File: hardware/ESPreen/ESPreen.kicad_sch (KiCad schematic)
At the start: 4 parts

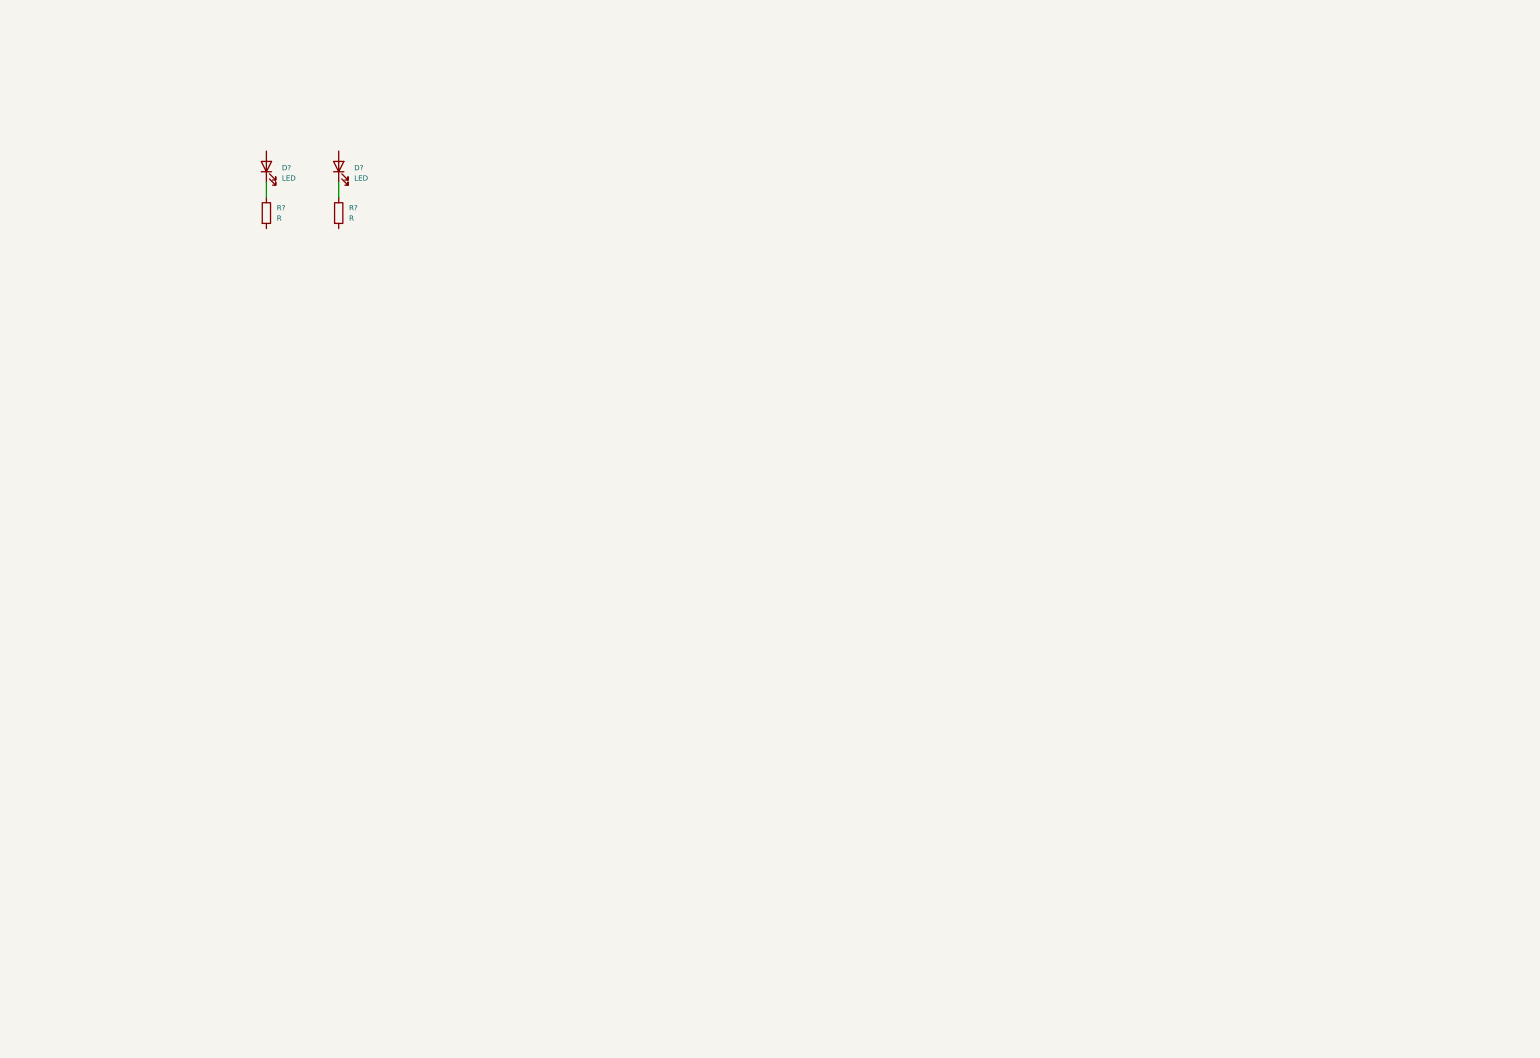
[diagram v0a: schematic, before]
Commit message: Update to finished board
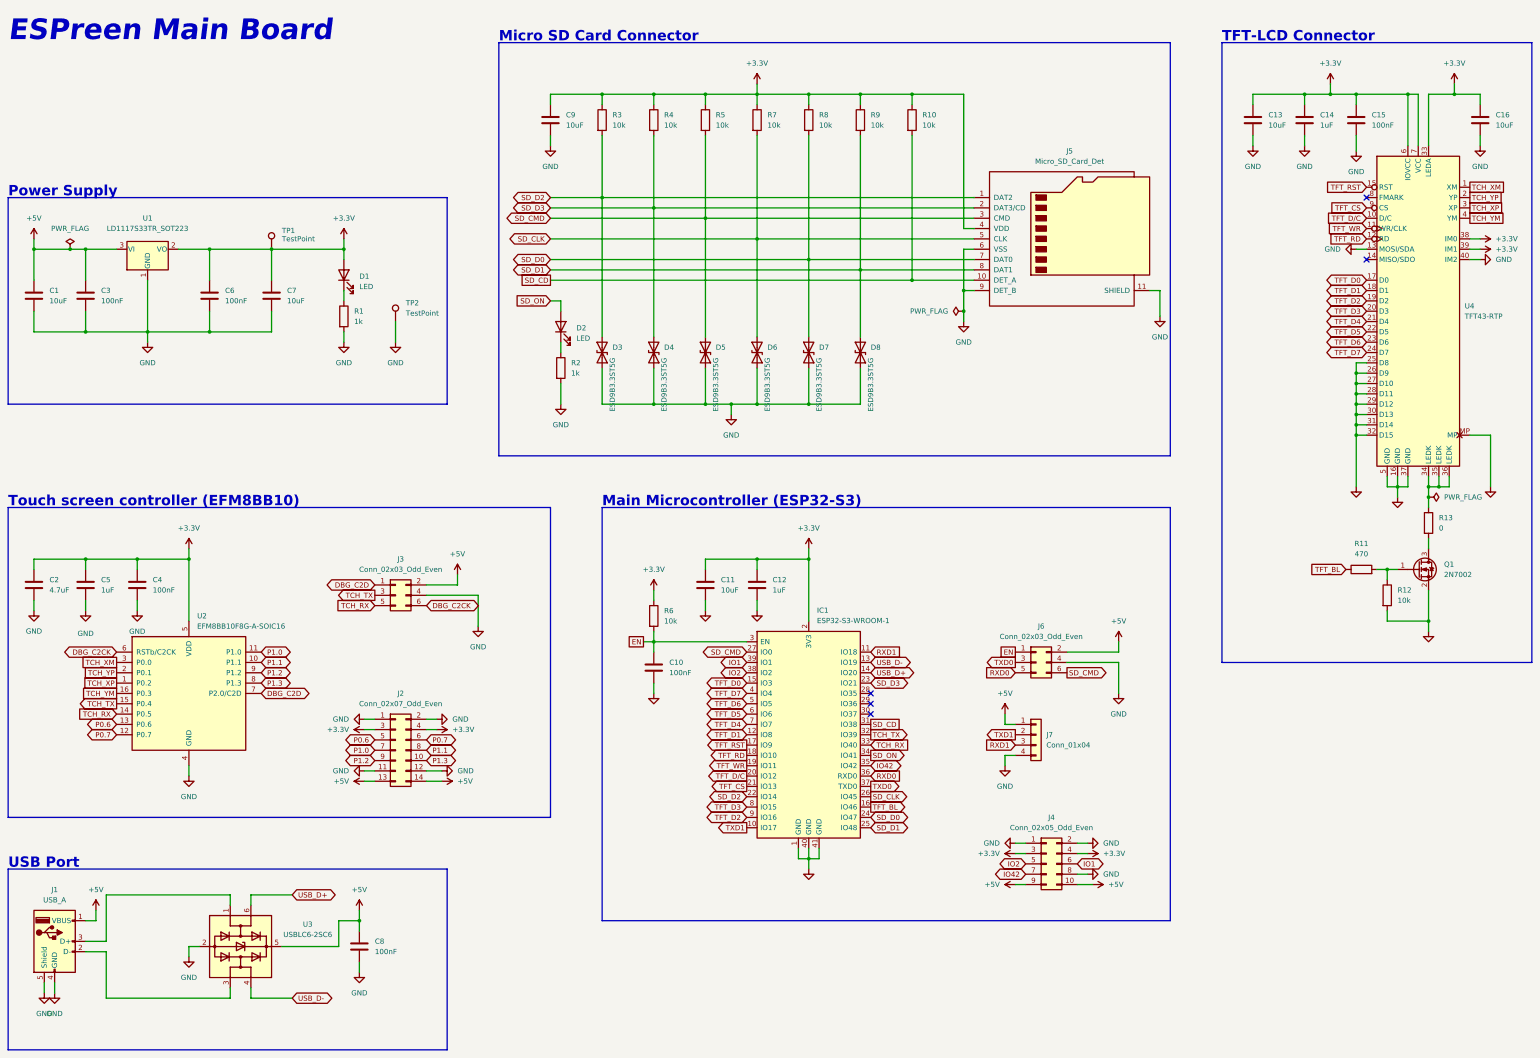
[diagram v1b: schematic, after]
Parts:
- added C1, C11, C13, C16, C7, C9: 10uF, Capacitor_SMD:C_0603_1608Metric_Pad1.08x0.95mm_HandSolder, symbol Device:C
- added C10, C15, C3, C4, C6, C8: 100nF, Capacitor_SMD:C_0603_1608Metric_Pad1.08x0.95mm_HandSolder, symbol Device:C
- added C12, C14, C5: 1uF, Capacitor_SMD:C_0603_1608Metric_Pad1.08x0.95mm_HandSolder, symbol Device:C
- added C2: 4.7uF, Capacitor_SMD:C_0603_1608Metric_Pad1.08x0.95mm_HandSolder, symbol Device:C
- added D3, D4, D5, D6, D7, D8: ESD9B3.3ST5G, Diode_SMD:D_SOD-523, symbol Diode:ESD9B3.3ST5G
- added IC1: ESP32-S3-WROOM-1, RF_Module:ESP32-S3-WROOM-1, symbol RF_Module2:ESP32-S3-WROOM-1
- added J1: USB_A, Connector_USB:USB_A_Molex_67643_Horizontal, symbol Connector:USB_A
- added J2: Conn_02x07_Odd_Even, Connector_PinHeader_2.54mm:PinHeader_2x07_P2.54mm_Vertical, symbol Connector_Generic:Conn_02x07_Odd_Even
- added J3, J6: Conn_02x03_Odd_Even, Connector_PinHeader_1.27mm+:PinHeader_2x03_P1.27mm_Vertical_Shrouded, symbol Connector_Generic:Conn_02x03_Odd_Even
- added J4: Conn_02x05_Odd_Even, Connector_PinHeader_2.54mm:PinHeader_2x05_P2.54mm_Vertical, symbol Connector_Generic:Conn_02x05_Odd_Even
- added J5: Micro_SD_Card_Det, Connector_Card+:microSD_XunPu-F115, symbol Connector:Micro_SD_Card_Det
- added J7: Conn_01x04, Connector_Molex+:Molex_SL_70553-0004_1x04_P2.54mm_Horizontal, symbol Connector_Generic:Conn_01x04
- added Q1: 2N7002, Package_TO_SOT_SMD:SOT-23, symbol Transistor_FET:2N7002
- added R10, R12, R3, R4, R5, R6, R7, R8, R9: 10k, Resistor_SMD:R_0603_1608Metric_Pad0.98x0.95mm_HandSolder, symbol Device:R
- added R11: 470, Resistor_SMD:R_0603_1608Metric_Pad0.98x0.95mm_HandSolder, symbol Device:R
- added R13: 0, Resistor_SMD:R_0603_1608Metric_Pad0.98x0.95mm_HandSolder, symbol Device:R
- added TP1, TP2: TestPoint, TestPoint:TestPoint_Pad_D1.0mm, symbol Connector:TestPoint
- added U1: LD1117S33TR_SOT223, Package_TO_SOT_SMD:SOT-223-3_TabPin2, symbol Regulator_Linear:LD1117S33TR_SOT223
- added U2: EFM8BB10F8G-A-SOIC16, Package_SO:SOIC-16_3.9x9.9mm_P1.27mm, symbol MCU_SiliconLabs:EFM8BB10F8G-A-SOIC16
- added U3: USBLC6-2SC6, Package_TO_SOT_SMD:SOT-23-6, symbol Power_Protection:USBLC6-2SC6
- added U4: TFT43-RTP, Connector_FFC-FPC+:Jushuo-AFC07-S40ECA-00_1x40-1MP_P0.50mm_Horizontal, symbol Display_Graphic+:TFT43-RTP
- D1, D2: renamed from D?; footprint (none) -> LED_SMD:LED_0603_1608Metric_Pad1.05x0.95mm_HandSolder
- R1, R2: renamed from R?; value R -> 1k; footprint (none) -> Resistor_SMD:R_0603_1608Metric_Pad0.98x0.95mm_HandSolder
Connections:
- net GND: now reaches R1.2
- net GND: now also R2.2, C1.2, C10.2, C11.2, C12.2, C13.2, C14.2, C15.2, C16.2, C2.2, C3.2, C4.2, C5.2, C6.2, C7.2, C8.2, C9.2, D3.1 (A1), D4.1 (A1), D5.1 (A1), D6.1 (A1), D7.1 (A1), D8.1 (A1), IC1.1 (GND), IC1.40 (GND), IC1.41 (GND), J1.4 (GND), J1.5 (Shield), J2.1 (Pin_1), J2.11 (Pin_11), J2.12 (Pin_12), J2.2 (Pin_2), J3.4 (Pin_4), J4.1 (Pin_1), J4.2 (Pin_2), J4.8 (Pin_8), J5.11 (SHIELD), J5.6 (VSS), J5.9 (DET_B), J6.4 (Pin_4), J7.4 (Pin_4), Q1.2 (S), R12.2, TP2.1, U1.1 (GND), U2.4 (GND), U3.2 (GND), U4.13 (MOSI/SDA), U4.16 (GND), U4.25 (D8), U4.26 (D9), U4.27 (D10), U4.28 (D11), U4.29 (D12), U4.30 (D13), U4.31 (D14), U4.32 (D15), U4.37 (GND), U4.40 (IM2), U4.5 (GND), U4.MP
- net SD_ON: now reaches D2.2 (A)
- net SD_ON: now also IC1.34 (IO41)
- net +3.3V: now reaches D1.2 (A)
- net +3.3V: now also C11.1, C12.1, C13.1, C14.1, C15.1, C16.1, C2.1, C4.1, C5.1, C6.1, C7.1, C9.1, IC1.2 (3V3), J2.3 (Pin_3), J2.4 (Pin_4), J4.3 (Pin_3), J4.4 (Pin_4), J5.4 (VDD), R10.1, R3.1, R4.1, R5.1, R6.1, R7.1, R8.1, R9.1, TP1.1, U1.2 (VO), U2.5 (VDD), U4.33 (LEDA), U4.38 (IM0), U4.39 (IM1), U4.6 (IOVCC), U4.7 (VCC)
- new net: J1.2 (D-), U3.3 (I/O2)
- new net: J1.3 (D+), U3.1 (I/O1)
- new net: R13.1, U4.34 (LEDK), U4.35 (LEDK), U4.36 (LEDK)
- new net: Q1.3 (D), R13.2
- new net: Q1.1 (G), R11.2, R12.1
- new net +5V: C1.1, C3.1, C8.1, J1.1 (VBUS), J2.13 (Pin_13), J2.14 (Pin_14), J3.2 (Pin_2), J4.10 (Pin_10), J4.9 (Pin_9), J6.2 (Pin_2), J7.1 (Pin_1), U1.3 (VI), U3.5 (VBUS)
- new net DBG_C2CK: J3.6 (Pin_6), U2.6 (RSTb/C2CK)
- new net DBG_C2D: J3.1 (Pin_1), U2.7 (P2.0/C2D)
- new net EN: C10.1, IC1.3 (EN), J6.1 (Pin_1), R6.2
- new net IO1: IC1.39 (IO1), J4.6 (Pin_6)
- new net IO2: IC1.38 (IO2), J4.5 (Pin_5)
- new net IO42: IC1.35 (IO42), J4.7 (Pin_7)
- new net P0.6: J2.5 (Pin_5), U2.13 (P0.6)
- new net P0.7: J2.6 (Pin_6), U2.12 (P0.7)
- new net P1.0: J2.7 (Pin_7), U2.11 (P1.0)
- new net P1.1: J2.8 (Pin_8), U2.10 (P1.1)
- new net P1.2: J2.9 (Pin_9), U2.9 (P1.2)
- new net P1.3: J2.10 (Pin_10), U2.8 (P1.3)
- new net RXD0: IC1.36 (RXD0), J6.5 (Pin_5)
- new net RXD1: IC1.11 (IO18), J7.3 (Pin_3)
- new net SD_CD: IC1.31 (IO38), J5.10 (DET_A), R10.2
- new net SD_CLK: D6.2 (A2), IC1.26 (IO45), J5.5 (CLK), R7.2
- new net SD_CMD: D5.2 (A2), IC1.27 (IO0), J5.3 (CMD), J6.6 (Pin_6), R5.2
- new net SD_D0: D7.2 (A2), IC1.24 (IO47), J5.7 (DAT0), R8.2
- new net SD_D1: D8.2 (A2), IC1.25 (IO48), J5.8 (DAT1), R9.2
- new net SD_D2: D3.2 (A2), IC1.22 (IO14), J5.1 (DAT2), R3.2
- new net SD_D3: D4.2 (A2), IC1.23 (IO21), J5.2 (DAT3/CD), R4.2
- new net TCH_RX: IC1.33 (IO40), J3.5 (Pin_5), U2.14 (P0.5)
- new net TCH_TX: IC1.32 (IO39), J3.3 (Pin_3), U2.15 (P0.4)
- new net TCH_XM: U2.3 (P0.0), U4.1 (XM)
- new net TCH_XP: U2.1 (P0.2), U4.3 (XP)
- new net TCH_YM: U2.16 (P0.3), U4.4 (YM)
- new net TCH_YP: U2.2 (P0.1), U4.2 (YP)
- new net TFT_BL: IC1.16 (IO46), R11.1
- new net TFT_CS: IC1.21 (IO13), U4.9 (CS)
- new net TFT_D0: IC1.15 (IO3), U4.17 (D0)
- new net TFT_D1: IC1.12 (IO8), U4.18 (D1)
- new net TFT_D2: IC1.9 (IO16), U4.19 (D2)
- new net TFT_D3: IC1.8 (IO15), U4.20 (D3)
- new net TFT_D4: IC1.7 (IO7), U4.21 (D4)
- new net TFT_D5: IC1.6 (IO6), U4.22 (D5)
- new net TFT_D6: IC1.5 (IO5), U4.23 (D6)
- new net TFT_D7: IC1.4 (IO4), U4.24 (D7)
- new net TFT_D/C: IC1.20 (IO12), U4.10 (D/C)
- new net TFT_RD: IC1.18 (IO10), U4.12 (RD)
- new net TFT_RST: IC1.17 (IO9), U4.15 (RST)
- new net TFT_WR: IC1.19 (IO11), U4.11 (WR/CLK)
- new net TXD0: IC1.37 (TXD0), J6.3 (Pin_3)
- new net TXD1: IC1.10 (IO17), J7.2 (Pin_2)
- new net USB_D+: IC1.14 (IO20), U3.6 (I/O1)
- new net USB_D-: IC1.13 (IO19), U3.4 (I/O2)
- no-connect marks 0 -> 5
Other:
- note added: "ESPreen Main Board"
- note added: "Main Microcontroller (ESP32-S3)"
- note added: "Micro SD Card Connector"
- note added: "Power Supply"
- note added: "TFT-LCD Connector"
- note added: "Touch screen controller (EFM8BB10)"
- note added: "USB Port"
- moved on the sheet: D1, D2, R1, R2
